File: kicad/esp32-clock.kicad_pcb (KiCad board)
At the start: 2 copper layers, 32.5 x 63 mm, 36 parts, among them J1 Battery Connector, P1 USB_C_Plug_USB2.0, SW1 RESET, SW2 BOOT, U1 ESP-12E, U2 CP2102N-Axx-xQFN20, U3 MCP73831-2-OT, U4 BCM857BS, U5 ME6211C12M5G-N

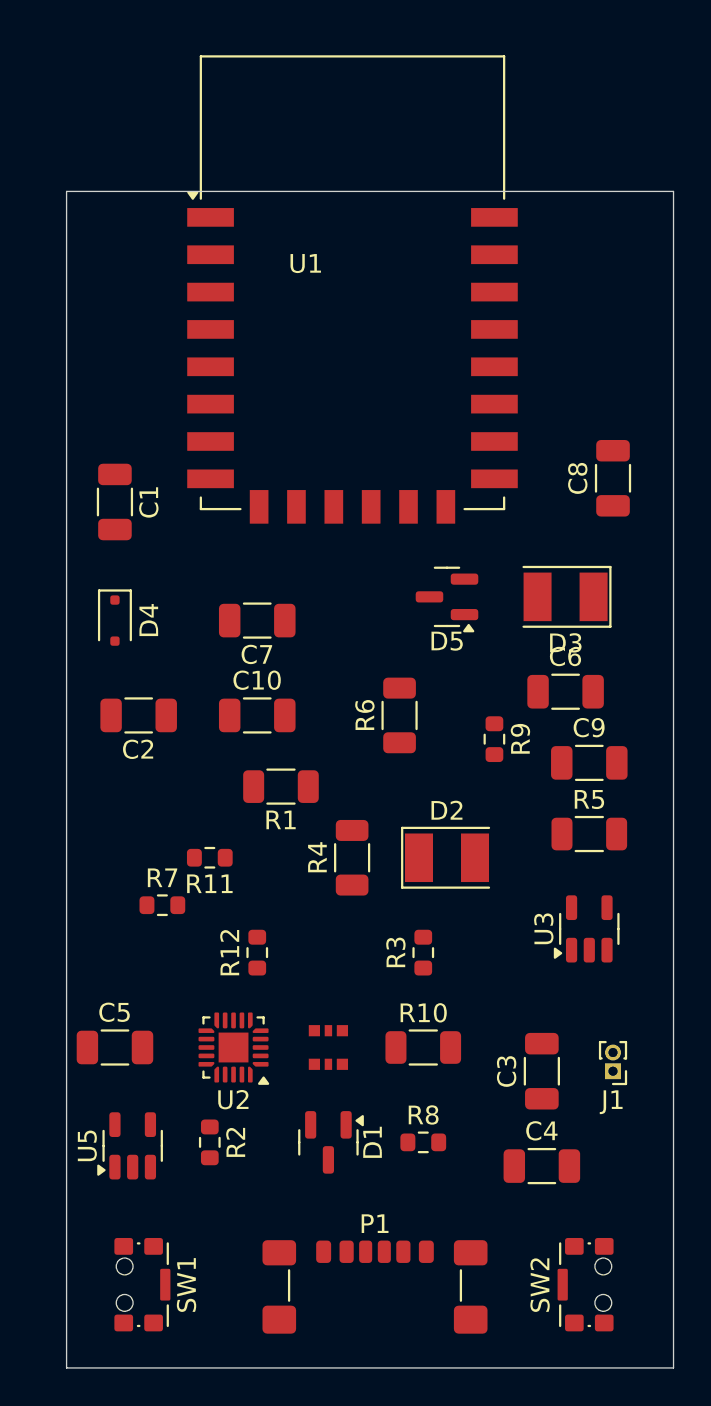
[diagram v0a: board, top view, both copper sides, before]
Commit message: init
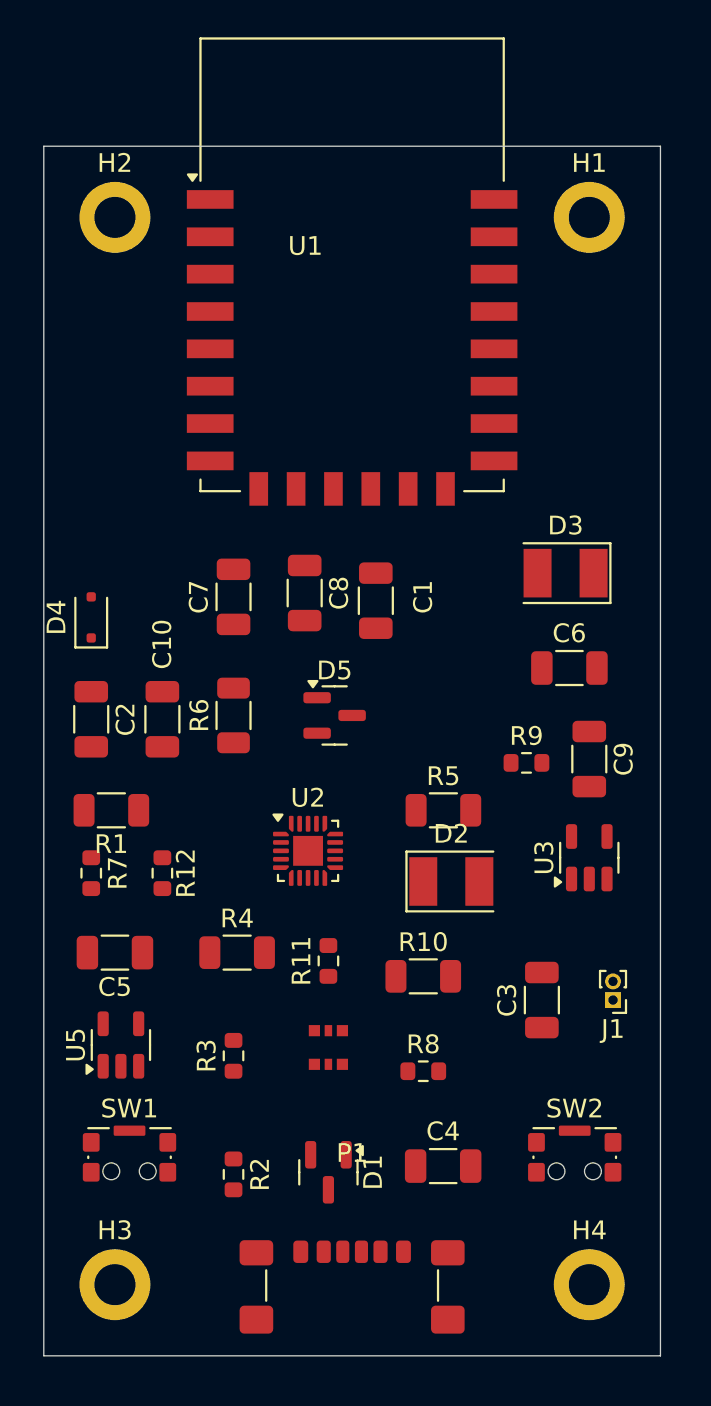
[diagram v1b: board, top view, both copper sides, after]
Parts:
- added H1: MountingHole, MountingHole:MountingHole_2.2mm_M2_DIN965_Pad, F.Cu at (110.5, 72.4)
- added H2: MountingHole, MountingHole:MountingHole_2.2mm_M2_DIN965_Pad, F.Cu at (85.1, 72.4)
- added H3: MountingHole, MountingHole:MountingHole_2.2mm_M2_DIN965_Pad, F.Cu at (85.1, 129.5)
- added H4: MountingHole, MountingHole:MountingHole_2.2mm_M2_DIN965_Pad, F.Cu at (110.5, 129.5)
- moved C8 17.6 mm to (95.2, 92.5), turned to -90 degrees
- moved C1 14.9 mm to (99.1, 92.9), turned to 90 degrees
- moved R3 11.6 mm to (91.4, 117.3)
- moved U2 11.3 mm to (95.4, 106.3), turned to 0 degrees
- moved R1 9.17 mm to (84.9, 104.1)
- moved R6 8.89 mm to (91.4, 99.1)
- moved D5 8.75 mm to (96.9, 99.1), turned to 0 degrees
- moved R11 8.42 mm to (96.5, 112.2), turned to 90 degrees
- moved R4 7.98 mm to (91.6, 111.8), turned to 0 degrees
- moved R5 7.92 mm to (102.7, 104.1)
- moved SW2 6.86 mm to (109.7, 122.7), turned to 0 degrees
- moved SW1 6.84 mm to (85.9, 122.7), turned to 0 degrees
- moved R12 6.63 mm to (87.6, 107.5)
- moved U5 5.44 mm to (85.4, 116.7)
- moved C4 5.28 mm to (102.7, 123.2)
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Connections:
- SW2 pad 2: unconnected-(SW2-Pad2) -> GND
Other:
- board size 32.5 x 63 mm -> 33 x 64.8 mm
